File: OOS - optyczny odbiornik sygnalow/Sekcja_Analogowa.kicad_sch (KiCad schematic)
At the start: 52 parts, among them J1 Conn_01x02_Socket, J2 Conn_01x02_Socket, J3 Conn_01x02_Socket, J4 Conn_01x02_Socket, J5 Conn_Coaxial, U1 OPA300AIDBVR, U2 OPA300AIDBVR

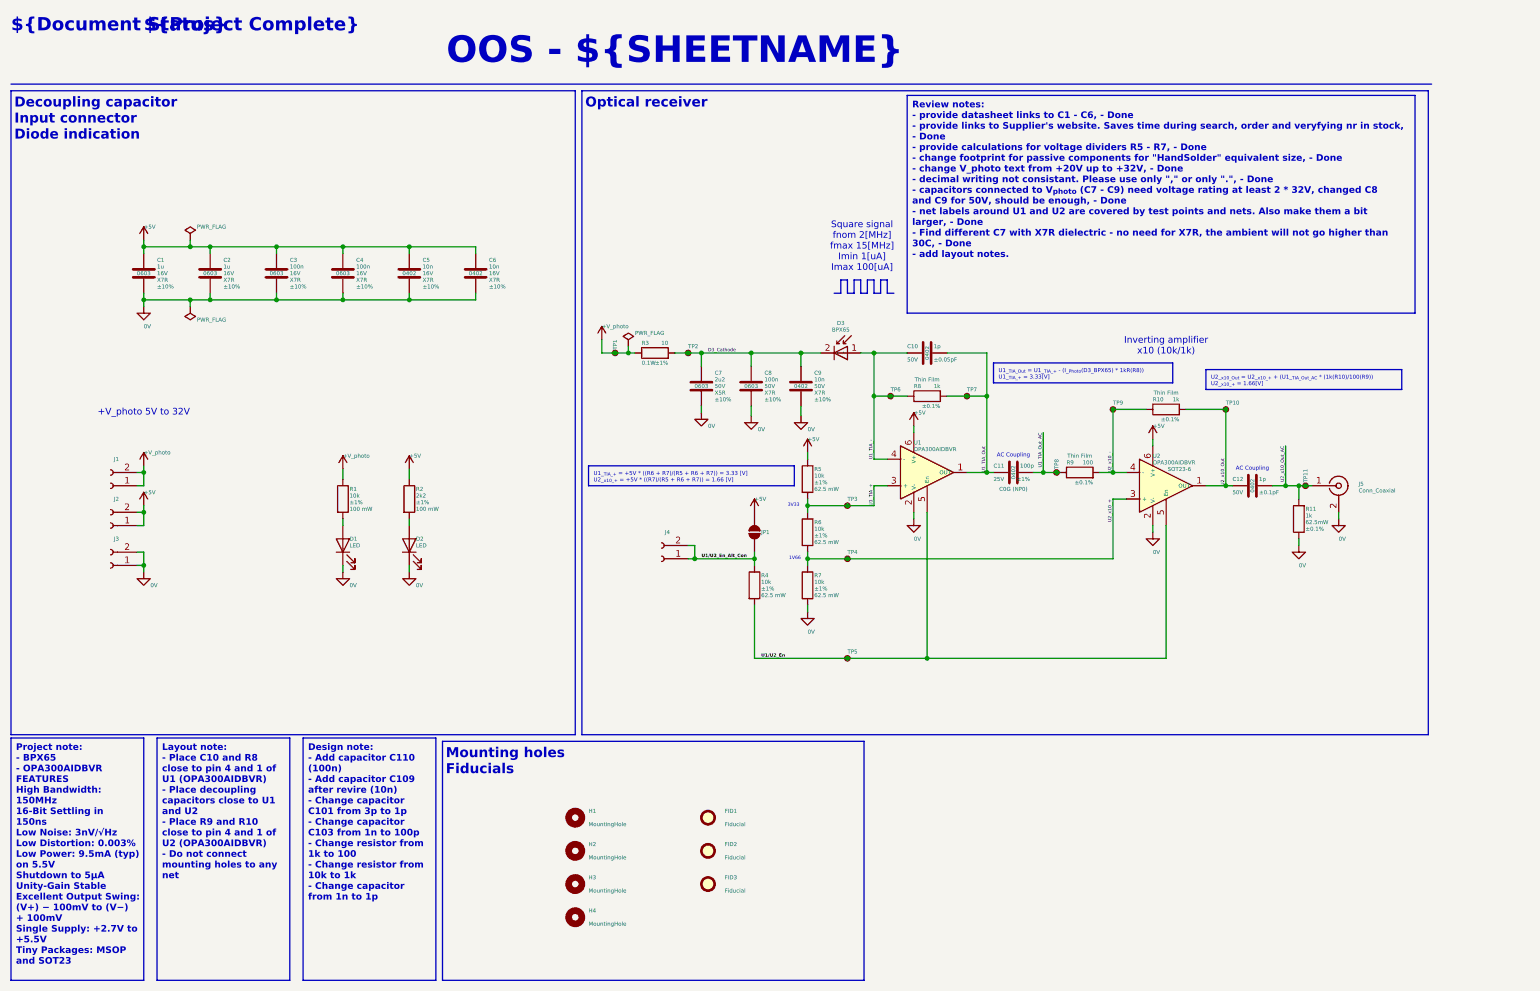
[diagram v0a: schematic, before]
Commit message: Finish Li-Lion section, add for review
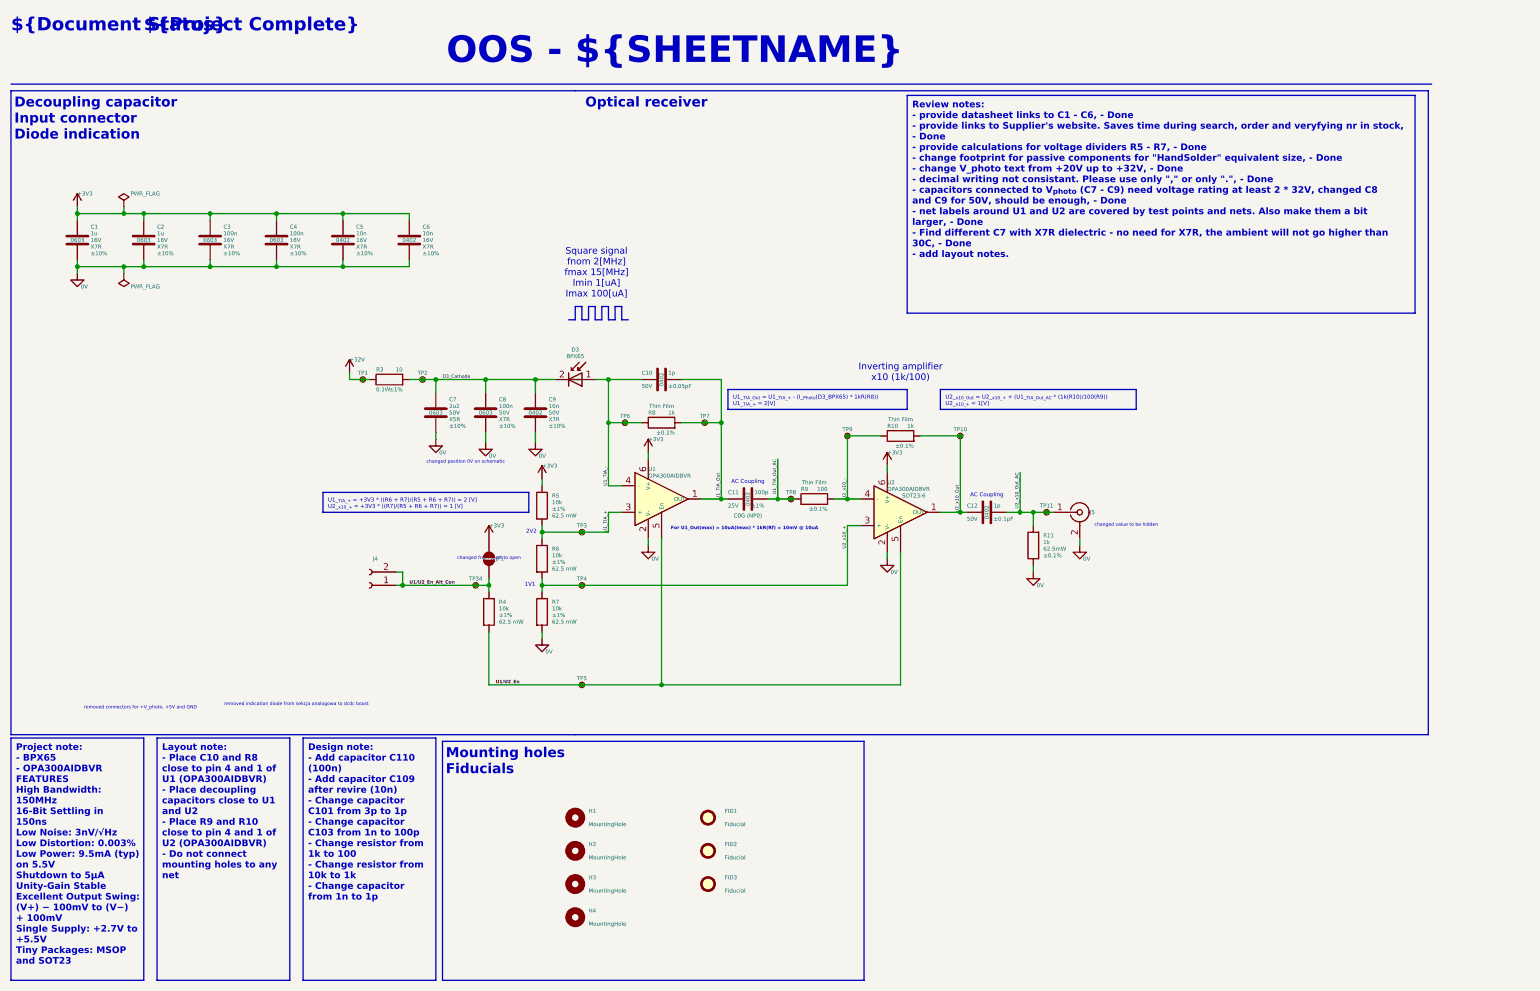
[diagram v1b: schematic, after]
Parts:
- removed D1, D2: LED, Diode_SMD:D_0603_1608Metric_Pad1.05x0.95mm_HandSolder, symbol Device:LED
- removed J1, J2, J3: Conn_01x02_Socket, Connector_PinHeader_2.54mm:PinHeader_1x02_P2.54mm_Vertical, symbol Connector:Conn_01x02_Socket
- removed R1: 10k, Resistor_SMD:R_0603_1608Metric_Pad0.98x0.95mm_HandSolder, symbol Device:R
- removed R2: 2k2, Resistor_SMD:R_0603_1608Metric_Pad0.98x0.95mm_HandSolder, symbol Device:R
- added TP34: TestPoint_Small, TestPoint:TestPoint_Pad_D1.0mm, symbol Connector:TestPoint_Small
- JP1: footprint Jumper:SolderJumper-2_P1.3mm_Bridged_RoundedPad1.0x1.5mm -> Jumper:SolderJumper-2_P1.3mm_Open_RoundedPad1.0x1.5mm
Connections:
- net U1/U2_En_Alt_Con: now also TP34.1
- net +5V renamed +3V3
- net +V_photo renamed +32V
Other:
- note added: "1V1"
- note added: "2V2"
- note added: "For U1_Out(max) = 10uA(Imax) * 1kR(Rf) = 10mV @ 10uA"
- note added: "Inverting amplifier x10 (1k/100)"
- note added: "changed from short to open"
- note added: "changed position 0V on schematic"
- note added: "changed value to be hidden"
- note added: "removed connectors for +V_photo, +5V and GND"
- note added: "removed indication diode from sekcja analogowa to dcdc boost"
- note removed: "+V_photo 5V to 32V"
- note removed: "1V66"
- note removed: "3V33"
- note removed: "Inverting amplifier x10 (10k/1k)"
- moved on the sheet: C1, C10, C11, C12, C2, C3, C4, C5, C6, C7, C8, C9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
